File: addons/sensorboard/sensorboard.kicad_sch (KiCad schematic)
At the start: 13 parts, among them J1 Conn_02x06_Odd_Even, J10 Adafruit_I2C_Header, J11 BME680_Header, J12 RGB_Header, J2 SparkFun_I2C_Header, J3 Adafruit_I2C_Header, J4 Pimoroni_I2CGarden_Header, J5 Pimoroni_I2CGarden_Header, J6 Adafruit_I2C_Header, J7 SparkFun_I2C_Header, J8 StemmaQT_Qwiic_Header, J9 StemmaQT_Qwiic_Header, U1 XIAO-RP2040

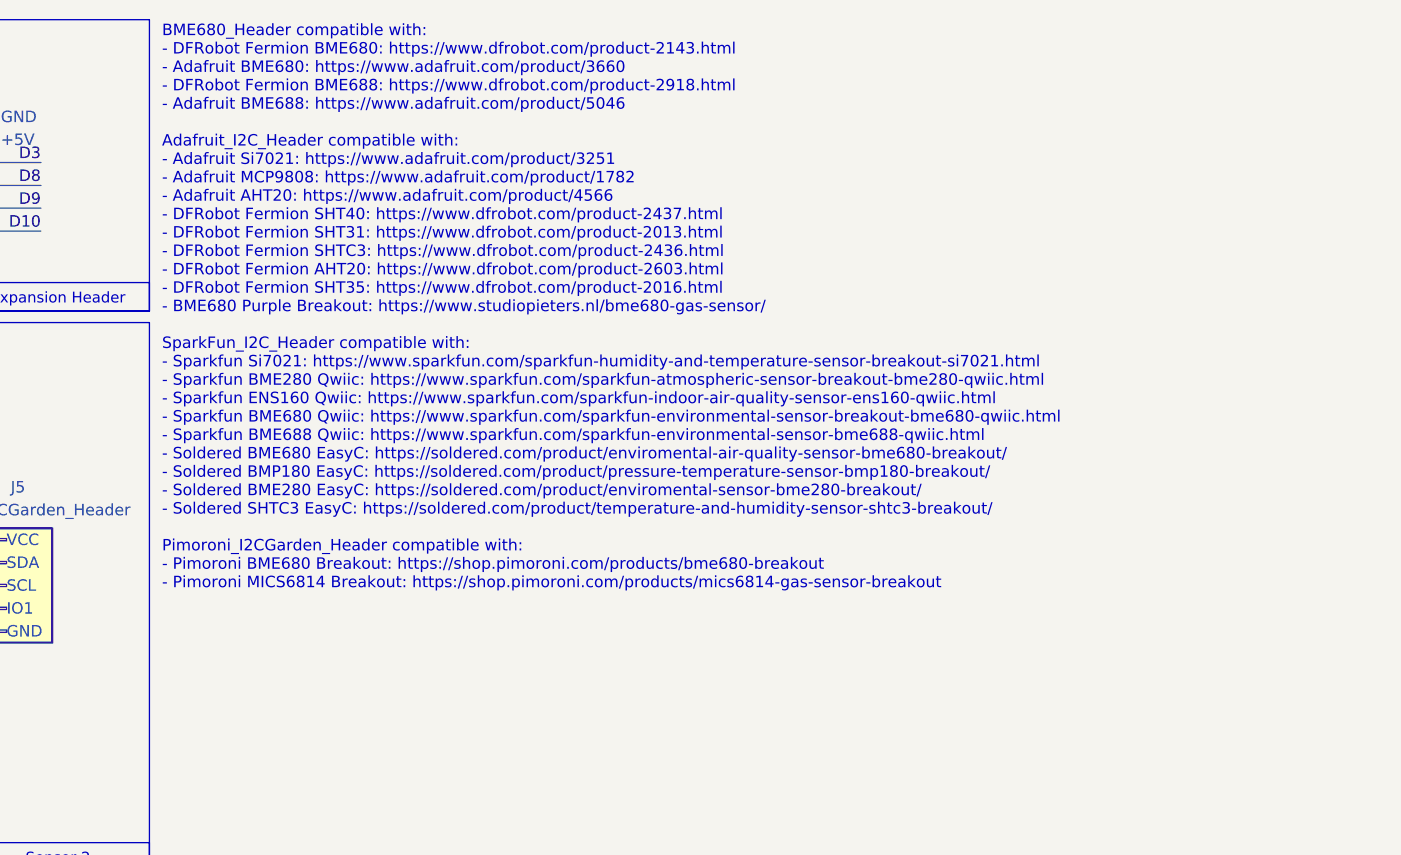
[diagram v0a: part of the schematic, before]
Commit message: Finalize aqstation
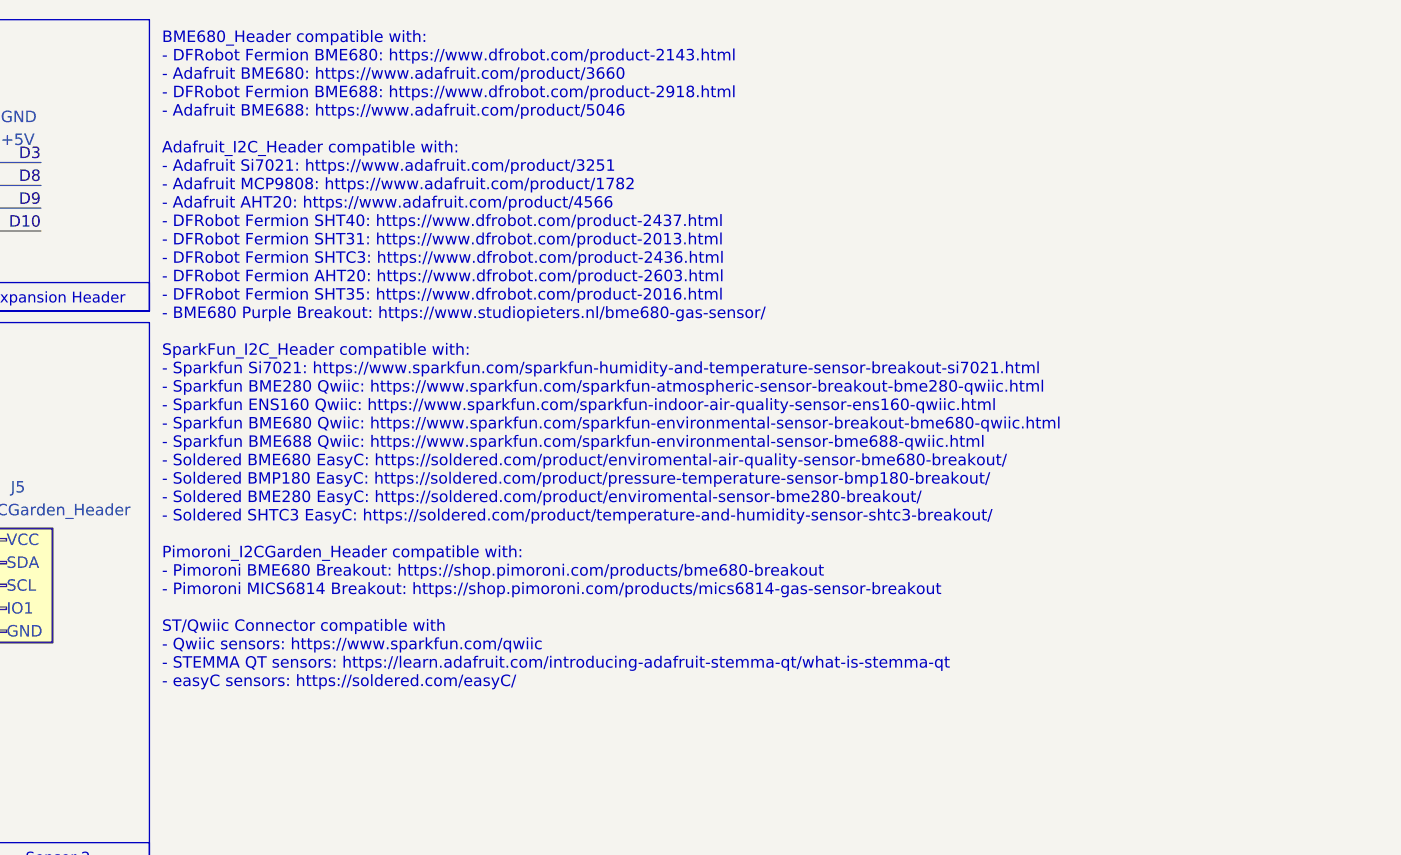
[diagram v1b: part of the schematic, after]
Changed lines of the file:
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@@
 		)
 	)
-	(text "BME680_Header compatible with:\n- DFRobot Fermion BME680: https://www.dfrobot.com/product-2143.html\n- Adafruit BME680: https://www.adafruit.com/product/3660\n- DFRobot Fermion BME688: https://www.dfrobot.com/product-2918.html\n- Adafruit BME688: https://www.adafruit.com/product/5046\n\nAdafruit_I2C_Header compatible with:\n- Adafruit Si7021: https://www.adafruit.com/product/3251\n- Adafruit MCP9808: https://www.adafruit.com/product/1782\n- Adafruit AHT20: https://www.adafruit.com/product/4566\n- DFRobot Fermion SHT40: https://www.dfrobot.com/product-2437.html\n- DFRobot Fermion SHT31: https://www.dfrobot.com/product-2013.html\n- DFRobot Fermion SHTC3: https://www.dfrobot.com/product-2436.html\n- DFRobot Fermion AHT20: https://www.dfrobot.com/product-2603.html\n- DFRobot Fermion SHT35: https://www.dfrobot.com/product-2016.html\n- BME680 Purple Breakout: https://www.studiopieters.nl/bme680-gas-sensor/\n\nSparkFun_I2C_Header compatible with:\n- Sparkfun Si7021: https://www.sparkfun.com/sparkfun-humidity-and-temperature-sensor-breakout-si7021.html\n- Sparkfun BME280 Qwiic: https://www.sparkfun.com/sparkfun-atmospheric-sensor-breakout-bme280-qwiic.html\n- Sparkfun ENS160 Qwiic: https://www.sparkfun.com/sparkfun-indoor-air-quality-sensor-ens160-qwiic.html\n- Sparkfun BME680 Qwiic: https://www.sparkfun.com/sparkfun-environmental-sensor-breakout-bme680-qwiic.html\n- Sparkfun BME688 Qwiic: https://www.sparkfun.com/sparkfun-environmental-sensor-bme688-qwiic.html\n- Soldered BME680 EasyC: https://soldered.com/product/enviromental-air-quality-sensor-bme680-breakout/\n- Soldered BMP180 EasyC: https://soldered.com/product/pressure-temperature-sensor-bmp180-breakout/\n- Soldered BME280 EasyC: https://soldered.com/product/enviromental-sensor-bme280-breakout/\n- Soldered SHTC3 EasyC: https://soldered.com/product/temperature-and-humidity-sensor-shtc3-breakout/\n\nPimoroni_I2CGarden_Header compatible with:\n- Pimoroni BME680 Breakout: https://shop.pimoroni.com/products/bme680-breakout\n- Pimoroni MICS6814 Breakout: https://shop.pimoroni.com/products/mics6814-gas-sensor-breakout"
+	(text "BME680_Header compatible with:\n- DFRobot Fermion BME680: https://www.dfrobot.com/product-2143.html\n- Adafruit BME680: https://www.adafruit.com/product/3660\n- DFRobot Fermion BME688: https://www.dfrobot.com/product-2918.html\n- Adafruit BME688: https://www.adafruit.com/product/5046\n\nAdafruit_I2C_Header compatible with:\n- Adafruit Si7021: https://www.adafruit.com/product/3251\n- Adafruit MCP9808: https://www.adafruit.com/product/1782\n- Adafruit AHT20: https://www.adafruit.com/product/4566\n- DFRobot Fermion SHT40: https://www.dfrobot.com/product-2437.html\n- DFRobot Fermion SHT31: https://www.dfrobot.com/product-2013.html\n- DFRobot Fermion SHTC3: https://www.dfrobot.com/product-2436.html\n- DFRobot Fermion AHT20: https://www.dfrobot.com/product-2603.html\n- DFRobot Fermion SHT35: https://www.dfrobot.com/product-2016.html\n- BME680 Purple Breakout: https://www.studiopieters.nl/bme680-gas-sensor/\n\nSparkFun_I2C_Header compatible with:\n- Sparkfun Si7021: https://www.sparkfun.com/sparkfun-humidity-and-temperature-sensor-breakout-si7021.html\n- Sparkfun BME280 Qwiic: https://www.sparkfun.com/sparkfun-atmospheric-sensor-breakout-bme280-qwiic.html\n- Sparkfun ENS160 Qwiic: https://www.sparkfun.com/sparkfun-indoor-air-quality-sensor-ens160-qwiic.html\n- Sparkfun BME680 Qwiic: https://www.sparkfun.com/sparkfun-environmental-sensor-breakout-bme680-qwiic.html\n- Sparkfun BME688 Qwiic: https://www.sparkfun.com/sparkfun-environmental-sensor-bme688-qwiic.html\n- Soldered BME680 EasyC: https://soldered.com/product/enviromental-air-quality-sensor-bme680-breakout/\n- Soldered BMP180 EasyC: https://soldered.com/product/pressure-temperature-sensor-bmp180-breakout/\n- Soldered BME280 EasyC: https://soldered.com/product/enviromental-sensor-bme280-breakout/\n- Soldered SHTC3 EasyC: https://soldered.com/product/temperature-and-humidity-sensor-shtc3-breakout/\n\nPimoroni_I2CGarden_Header compatible with:\n- Pimoroni BME680 Breakout: https://shop.pimoroni.com/products/bme680-breakout\n- Pimoroni MICS6814 Breakout: https://shop.pimoroni.com/products/mics6814-gas-sensor-breakout\n\nST/Qwiic Connector compatible with\n- Qwiic sensors: https://www.sparkfun.com/qwiic\n- STEMMA QT sensors: https://learn.adafruit.com/introducing-adafruit-stemma-qt/what-is-stemma-qt\n- easyC sensors: https://soldered.com/easyC/"
 		(exclude_from_sim no)
-		(at 131.572 13.97 0)
+		(at 131.572 14.732 0)
 		(effects
 			(font
